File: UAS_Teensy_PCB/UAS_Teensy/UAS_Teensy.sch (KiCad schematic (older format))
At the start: 8 parts, among them J1 UAS-rescue_SM02B-PASS-TBT(LF)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, J2 SM04B-GHS-TB(LF)(SN)-, J3 SM07B-GHS-TB(LF)(SN), J4 SM07B-GHS-TB(LF)(SN), J5 SM04B-GHS-TB(LF)(SN)-, J6 SM04B-GHS-TB(LF)(SN)-, J7 SM04B-GHS-TB(LF)(SN)-, U1 Teensy4.0

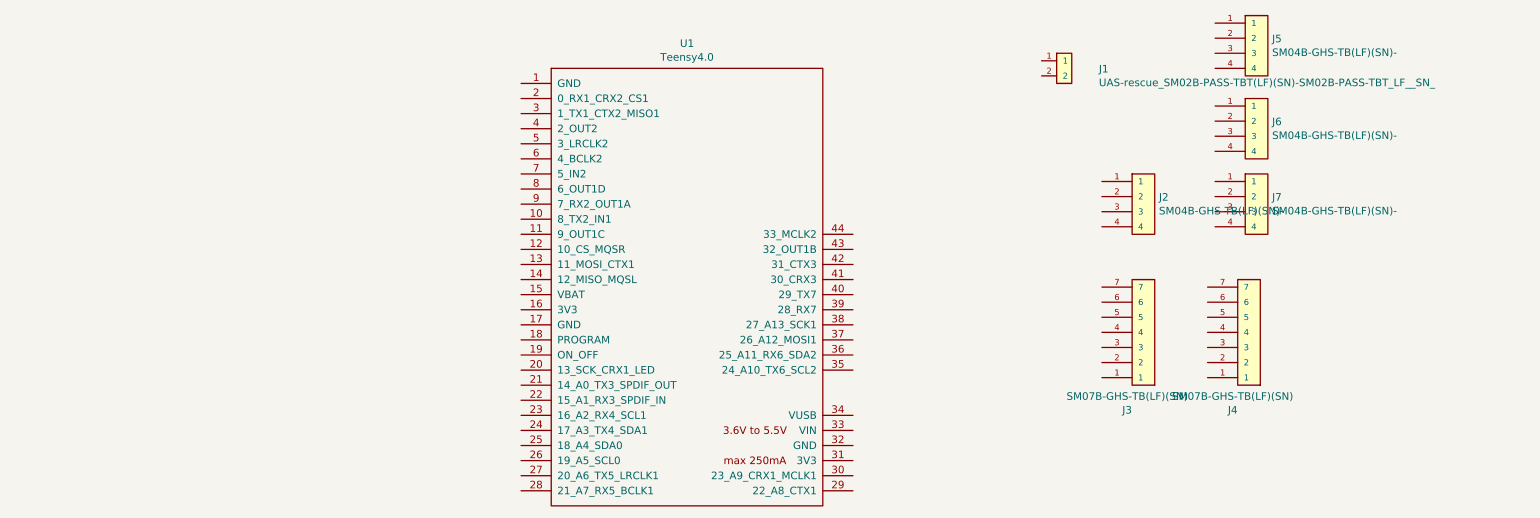
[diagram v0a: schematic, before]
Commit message: Schematic Wiring V1
First Step in Schematic Wiring
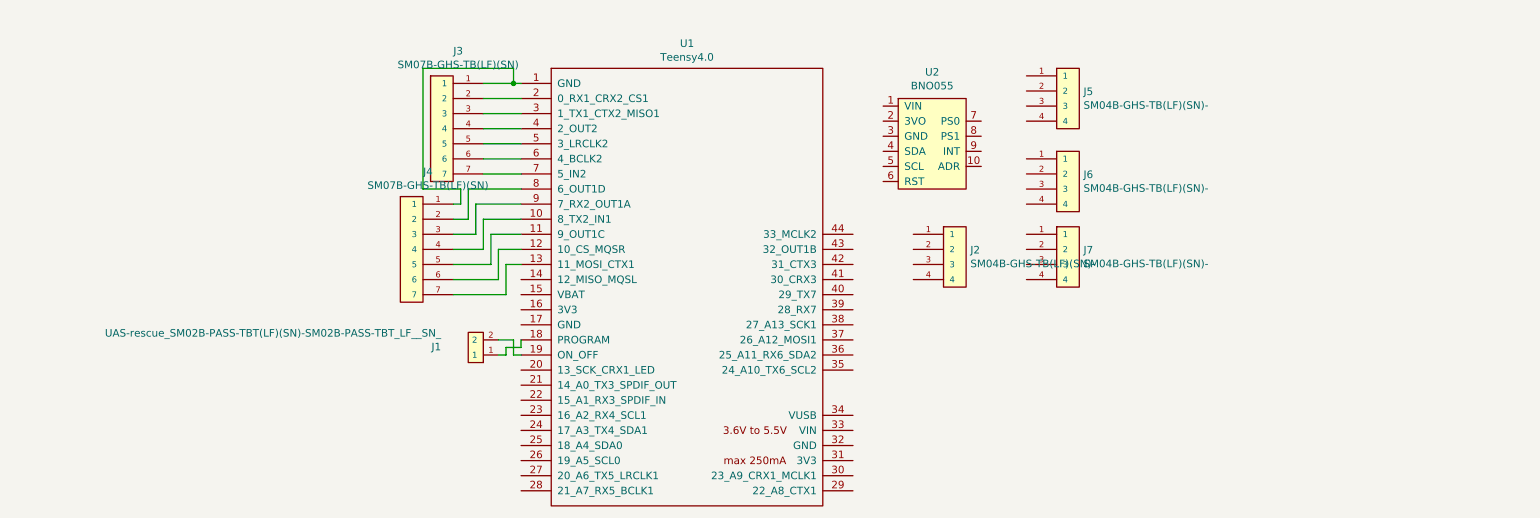
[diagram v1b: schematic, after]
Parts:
- added U2: BNO055, UAS_Teensy:BNO055_Breakout, symbol UAS_Teensy:BNO055
- J1: footprint JST_SM02B-PASS-TBT(LF)(SN) -> UAS_Teensy:SM02BGHSTBLFSN
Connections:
- net at U1.1 (GND): now also J3.1, J4.1
- net at U1.10 (8_TX2_IN1): now also J4.4
- net at U1.11 (9_OUT1C): now also J4.5
- net at U1.12 (10_CS_MQSR): now also J4.6
- net at U1.13 (11_MOSI_CTX1): now also J4.7
- net at U1.18 (PROGRAM): now also J1.1
- net at U1.19 (ON_OFF): now also J1.2
- net at U1.2 (0_RX1_CRX2_CS1): now also J3.2
- net at U1.3 (1_TX1_CTX2_MISO1): now also J3.3
- net at U1.4 (2_OUT2): now also J3.4
- net at U1.5 (3_LRCLK2): now also J3.5
- net at U1.6 (4_BCLK2): now also J3.6
- net at U1.7 (5_IN2): now also J3.7
- net at U1.8 (6_OUT1D): now also J4.2
- net at U1.9 (7_RX2_OUT1A): now also J4.3
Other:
- moved on the sheet: J1, J2, J3, J4, J5, J6, J7
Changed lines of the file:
@@
 L UAS:SM04B-GHS-TB(LF)(SN)- J2
 U 1 1 6073EDF2
-P 8400 2250
-F 0 "J2" H 8378 2346 50  0000 L CNN
-F 1 "SM04B-GHS-TB(LF)(SN)-" H 8378 2255 50  0000 L CNN
-F 2 "JST_SM04B-GHS-TB(LF)(SN)-" H 8400 2250 50  0001 L BNN
-F 3 "" H 8400 2250 50  0001 L BNN
-F 4 "NA" H 8400 2250 50  0001 L BNN "PARTREV"
-F 5 "Manufacturer Recommendations" H 8400 2250 50  0001 L BNN "STANDARD"
-F 6 "JHS" H 8400 2250 50  0001 L BNN "MANUFACTURER"
-	1    8400 2250
+P 7150 2600
+F 0 "J2" H 7128 2696 50  0000 L CNN
+F 1 "SM04B-GHS-TB(LF)(SN)-" H 7128 2605 50  0000 L CNN
+F 2 "JST_SM04B-GHS-TB(LF)(SN)-" H 7150 2600 50  0001 L BNN
+F 3 "" H 7150 2600 50  0001 L BNN
+F 4 "NA" H 7150 2600 50  0001 L BNN "PARTREV"
+F 5 "Manufacturer Recommendations" H 7150 2600 50  0001 L BNN "STANDARD"
+F 6 "JHS" H 7150 2600 50  0001 L BNN "MANUFACTURER"
+	1    7150 2600
 	1    0    0    -1
 $EndComp
@@
 L UAS:SM07B-GHS-TB(LF)(SN) J3
 U 1 1 6073F50A
-P 8400 2950
-F 0 "J3" H 8633 3565 50  0000 C CNN
-F 1 "SM07B-GHS-TB(LF)(SN)" H 8633 3474 50  0000 C CNN
-F 2 "JST_SM07B-GHS-TB(LF)(SN)" H 8400 2950 50  0001 L BNN
-F 3 "" H 8400 2950 50  0001 L BNN
-F 4 "MANUFACTURER STANDARD" H 8400 2950 50  0001 L BNN "STANDARD"
-F 5 "JST" H 8400 2950 50  0001 L BNN "MANUFACTURER"
-F 6 "NA" H 8400 2950 50  0001 L BNN "PARTREV"
-	1    8400 2950
-	-1   0    0    1
+P 3500 1800
+F 0 "J3" H 3733 2415 50  0000 C CNN
+F 1 "SM07B-GHS-TB(LF)(SN)" H 3733 2324 50  0000 C CNN
+F 2 "JST_SM07B-GHS-TB(LF)(SN)" H 3500 1800 50  0001 L BNN
+F 3 "" H 3500 1800 50  0001 L BNN
+F 4 "MANUFACTURER STANDARD" H 3500 1800 50  0001 L BNN "STANDARD"
+F 5 "JST" H 3500 1800 50  0001 L BNN "MANUFACTURER"
+F 6 "NA" H 3500 1800 50  0001 L BNN "PARTREV"
+	1    3500 1800
+	1    0    0    -1
 $EndComp
 $Comp
 L UAS:SM07B-GHS-TB(LF)(SN) J4
 U 1 1 60740985
-P 9100 2950
-F 0 "J4" H 9333 3565 50  0000 C CNN
-F 1 "SM07B-GHS-TB(LF)(SN)" H 9333 3474 50  0000 C CNN
-F 2 "JST_SM07B-GHS-TB(LF)(SN)" H 9100 2950 50  0001 L BNN
-F 3 "" H 9100 2950 50  0001 L BNN
-F 4 "MANUFACTURER STANDARD" H 9100 2950 50  0001 L BNN "STANDARD"
-F 5 "JST" H 9100 2950 50  0001 L BNN "MANUFACTURER"
-F 6 "NA" H 9100 2950 50  0001 L BNN "PARTREV"
-	1    9100 2950
-	-1   0    0    1
+P 3300 2600
+F 0 "J4" H 3533 3215 50  0000 C CNN
+F 1 "SM07B-GHS-TB(LF)(SN)" H 3533 3124 50  0000 C CNN
+F 2 "JST_SM07B-GHS-TB(LF)(SN)" H 3300 2600 50  0001 L BNN
+F 3 "" H 3300 2600 50  0001 L BNN
+F 4 "MANUFACTURER STANDARD" H 3300 2600 50  0001 L BNN "STANDARD"
+F 5 "JST" H 3300 2600 50  0001 L BNN "MANUFACTURER"
+F 6 "NA" H 3300 2600 50  0001 L BNN "PARTREV"
+	1    3300 2600
+	1    0    0    -1
 $EndComp
 $Comp
 L UAS:SM04B-GHS-TB(LF)(SN)- J5
 U 1 1 60740F72
-P 9150 1200
-F 0 "J5" H 9128 1296 50  0000 L CNN
-F 1 "SM04B-GHS-TB(LF)(SN)-" H 9128 1205 50  0000 L CNN
-F 2 "JST_SM04B-GHS-TB(LF)(SN)-" H 9150 1200 50  0001 L BNN
-F 3 "" H 9150 1200 50  0001 L BNN
-F 4 "NA" H 9150 1200 50  0001 L BNN "PARTREV"
-F 5 "Manufacturer Recommendations" H 9150 1200 50  0001 L BNN "STANDARD"
-F 6 "JHS" H 9150 1200 50  0001 L BNN "MANUFACTURER"
-	1    9150 1200
+P 7900 1550
+F 0 "J5" H 7878 1646 50  0000 L CNN
+F 1 "SM04B-GHS-TB(LF)(SN)-" H 7878 1555 50  0000 L CNN
+F 2 "JST_SM04B-GHS-TB(LF)(SN)-" H 7900 1550 50  0001 L BNN
+F 3 "" H 7900 1550 50  0001 L BNN
+F 4 "NA" H 7900 1550 50  0001 L BNN "PARTREV"
+F 5 "Manufacturer Recommendations" H 7900 1550 50  0001 L BNN "STANDARD"
+F 6 "JHS" H 7900 1550 50  0001 L BNN "MANUFACTURER"
+	1    7900 1550
 	1    0    0    -1
 $EndComp
@@
 L UAS:SM04B-GHS-TB(LF)(SN)- J6
 U 1 1 60741E63
-P 9150 1750
-F 0 "J6" H 9128 1846 50  0000 L CNN
-F 1 "SM04B-GHS-TB(LF)(SN)-" H 9128 1755 50  0000 L CNN
-F 2 "JST_SM04B-GHS-TB(LF)(SN)-" H 9150 1750 50  0001 L BNN
-F 3 "" H 9150 1750 50  0001 L BNN
-F 4 "NA" H 9150 1750 50  0001 L BNN "PARTREV"
-F 5 "Manufacturer Recommendations" H 9150 1750 50  0001 L BNN "STANDARD"
-F 6 "JHS" H 9150 1750 50  0001 L BNN "MANUFACTURER"
-	1    9150 1750
+P 7900 2100
+F 0 "J6" H 7878 2196 50  0000 L CNN
+F 1 "SM04B-GHS-TB(LF)(SN)-" H 7878 2105 50  0000 L CNN
+F 2 "JST_SM04B-GHS-TB(LF)(SN)-" H 7900 2100 50  0001 L BNN
+F 3 "" H 7900 2100 50  0001 L BNN
+F 4 "NA" H 7900 2100 50  0001 L BNN "PARTREV"
+F 5 "Manufacturer Recommendations" H 7900 2100 50  0001 L BNN "STANDARD"
+F 6 "JHS" H 7900 2100 50  0001 L BNN "MANUFACTURER"
+	1    7900 2100
 	1    0    0    -1
 $EndComp
@@
 L UAS:SM04B-GHS-TB(LF)(SN)- J7
 U 1 1 60742445
-P 9150 2250
-F 0 "J7" H 9128 2346 50  0000 L CNN
-F 1 "SM04B-GHS-TB(LF)(SN)-" H 9128 2255 50  0000 L CNN
-F 2 "JST_SM04B-GHS-TB(LF)(SN)-" H 9150 2250 50  0001 L BNN
-F 3 "" H 9150 2250 50  0001 L BNN
-F 4 "NA" H 9150 2250 50  0001 L BNN "PARTREV"
-F 5 "Manufacturer Recommendations" H 9150 2250 50  0001 L BNN "STANDARD"
-F 6 "JHS" H 9150 2250 50  0001 L BNN "MANUFACTURER"
-	1    9150 2250
+P 7900 2600
+F 0 "J7" H 7878 2696 50  0000 L CNN
+F 1 "SM04B-GHS-TB(LF)(SN)-" H 7878 2605 50  0000 L CNN
+F 2 "JST_SM04B-GHS-TB(LF)(SN)-" H 7900 2600 50  0001 L BNN
+F 3 "" H 7900 2600 50  0001 L BNN
+F 4 "NA" H 7900 2600 50  0001 L BNN "PARTREV"
+F 5 "Manufacturer Recommendations" H 7900 2600 50  0001 L BNN "STANDARD"
+F 6 "JHS" H 7900 2600 50  0001 L BNN "MANUFACTURER"
+	1    7900 2600
 	1    0    0    -1
 $EndComp
@@
 L UAS:UAS-rescue_SM02B-PASS-TBT(LF)(SN)-SM02B-PASS-TBT_LF__SN_ J1
 U 1 1 60742753
-P 7750 1300
-F 0 "J1" H 7980 1296 50  0000 L CNN
-F 1 "UAS-rescue_SM02B-PASS-TBT(LF)(SN)-SM02B-PASS-TBT_LF__SN_" H 7980 1205 50  0000 L CNN
-F 2 "JST_SM02B-PASS-TBT(LF)(SN)" H 7750 1300 50  0001 L BNN
-F 3 "" H 7750 1300 50  0001 L BNN
-F 4 "N/A" H 7750 1300 50  0001 L BNN "PARTREV"
-F 5 "JST" H 7750 1300 50  0001 L BNN "MANUFACTURER"
-F 6 "Manufacturer Recommendations" H 7750 1300 50  0001 L BNN "STANDARD"
-F 7 "5.7 mm" H 7750 1300 50  0001 L BNN "MAXIMUM_PACKAGE_HEIGHT"
-	1    7750 1300
+P 3850 3150
+F 0 "J1" H 4080 3146 50  0000 L CNN
+F 1 "UAS-rescue_SM02B-PASS-TBT(LF)(SN)-SM02B-PASS-TBT_LF__SN_" H 4080 3055 50  0000 L CNN
+F 2 "UAS_Teensy:SM02BGHSTBLFSN" H 3850 3150 50  0001 L BNN
+F 3 "" H 3850 3150 50  0001 L BNN
+F 4 "N/A" H 3850 3150 50  0001 L BNN "PARTREV"
+F 5 "JST" H 3850 3150 50  0001 L BNN "MANUFACTURER"
+F 6 "Manufacturer Recommendations" H 3850 3150 50  0001 L BNN "STANDARD"
+F 7 "5.7 mm" H 3850 3150 50  0001 L BNN "MAXIMUM_PACKAGE_HEIGHT"
+	1    3850 3150
+	-1   0    0    1
+$EndComp
+Wire Wire Line
+	3700 2200 3750 2200
+Wire Wire Line
+	3750 2200 3750 2100
+Wire Wire Line
+	3750 2100 3500 2100
+Wire Wire Line
+	3500 2100 3500 1300
+Wire Wire Line
+	3500 1300 4100 1300
+Wire Wire Line
+	4100 1300 4100 1400
+Wire Wire Line
+	4100 1400 4150 1400
+Wire Wire Line
+	3900 1400 4100 1400
+Connection ~ 4100 1400
+Wire Wire Line
+	3700 2300 3800 2300
+Wire Wire Line
+	3800 2300 3800 2100
+Wire Wire Line
+	3800 2100 4150 2100
+Wire Wire Line
+	3700 2400 3850 2400
+Wire Wire Line
+	3850 2400 3850 2200
+Wire Wire Line
+	3850 2200 4150 2200
+Wire Wire Line
+	4150 2300 3900 2300
+Wire Wire Line
+	3900 2300 3900 2500
+Wire Wire Line
+	3900 2500 3700 2500
+Wire Wire Line
+	4150 2400 3950 2400
+Wire Wire Line
+	3950 2400 3950 2600
+Wire Wire Line
+	3950 2600 3700 2600
+Wire Wire Line
+	3700 2700 4000 2700
+Wire Wire Line
+	4000 2700 4000 2500
+Wire Wire Line
+	4000 2500 4150 2500
+Wire Wire Line
+	3700 2800 4050 2800
+Wire Wire Line
+	4050 2800 4050 2600
+Wire Wire Line
+	4050 2600 4150 2600
+Wire Wire Line
+	4150 1500 3900 1500
+Wire Wire Line
+	3900 1600 4150 1600
+Wire Wire Line
+	4150 1700 3900 1700
+Wire Wire Line
+	3900 1800 4150 1800
+Wire Wire Line
+	4150 1900 3900 1900
+Wire Wire Line
+	3900 2000 4150 2000
+$Comp
+L UAS_Teensy:BNO055 U2
+U 1 1 6074FC0F
+P 6900 1800
+F 0 "U2" H 6875 2275 50  0000 C CNN
+F 1 "BNO055" H 6875 2184 50  0000 C CNN
+F 2 "UAS_Teensy:BNO055_Breakout" H 6900 2350 50  0001 C CNN
+F 3 "" H 6900 2350 50  0001 C CNN
+	1    6900 1800
 	1    0    0    -1
 $EndComp
+Wire Wire Line
+	4000 3100 4100 3100
+Wire Wire Line
+	4100 3100 4100 3200
+Wire Wire Line
+	4100 3200 4150 3200
+Wire Wire Line
+	4000 3200 4050 3200
+Wire Wire Line
+	4050 3200 4050 3150
+Wire Wire Line
+	4050 3150 4150 3150
+Wire Wire Line
+	4150 3150 4150 3100
 $EndSCHEMATC
